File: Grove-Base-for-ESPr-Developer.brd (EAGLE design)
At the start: 26 x 26 mm, 8 parts, among them J1 4P-2.0, J2 4P-2.0, J3 4P-2.0, J4 4P-2.0

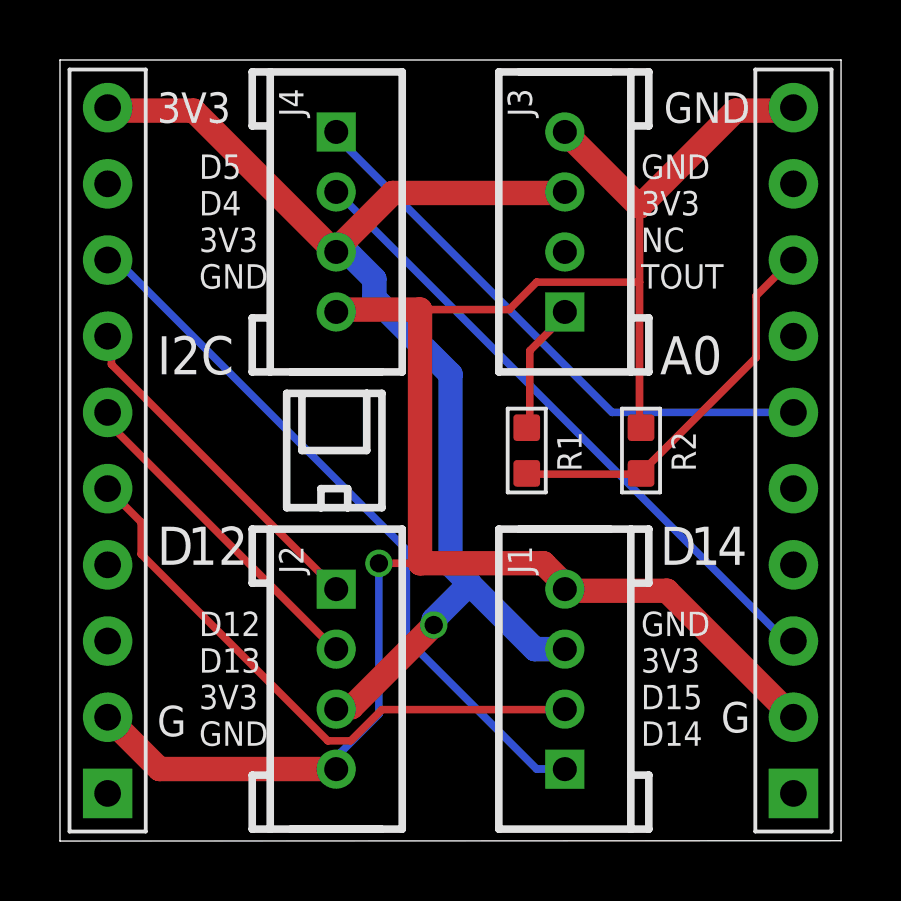
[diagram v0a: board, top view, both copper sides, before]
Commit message: 1st 5V evt
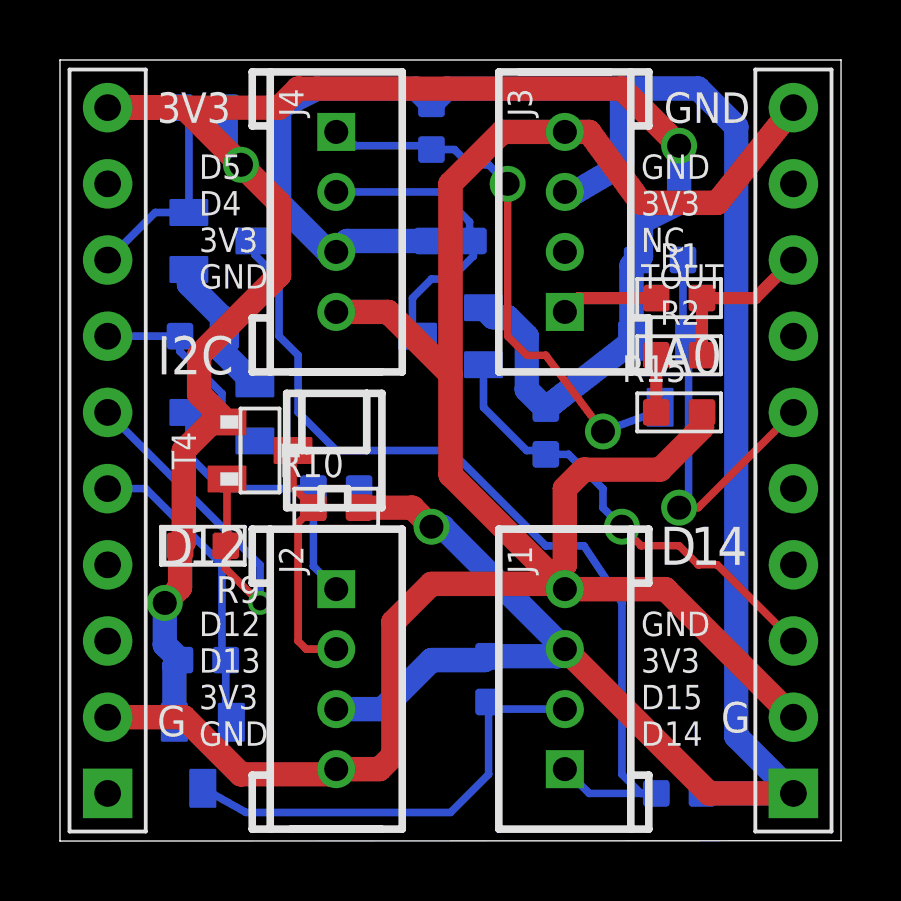
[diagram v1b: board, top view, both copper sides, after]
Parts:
- added R10, R11, R12, R13, R14, R3, R4, R5, R6, R7, R8, R9: 1K, Seeed-OPL-Resistor:R0603
- added R15: 27K, Seeed-OPL-Resistor:R0603
- added T1, T2, T3, T4, T5, T6: (no value), we-transistor:SOT23
- R1: value 220K -> 200K
- R2: value 100K -> 24K
- moved R1 7.18 mm to (20.3, 17.8), turned to 270 degrees
- moved R2 3.42 mm to (20.3, 15.9), turned to 90 degrees
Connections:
- new net IO12_5V: J2.1, R8.1, T3.3
- new net IO13_5V: J2.2, R10.2, T4.3
- new net IO14_5V: J1.1, R4.2, T1.3
- new net IO15_5V: J1.2, R6.2, T2.3
- new net IO4_5V: J4.2, R14.2, T6.3
- new net IO5_5V: J4.1, R12.1, T5.3
- new net N$6: R15.2, R2.1
- net 3V3: now also R11.2, R13.1, R3.1, R5.1, R7.2, R9.1, T1.1, T2.1, T3.1, T4.1, T5.1, T6.1; no longer J1.3, J2.3, J3.3, J4.3
- net 5V: now also J1.3, J2.3, J3.3, J4.3, R10.1, R12.2, R14.1, R4.1, R6.1, R8.2
- net GND: now also R15.1; no longer R2.1
- net IO12: now also R7.1, T3.2; no longer J2.1
- net IO13: now also R9.2, T4.2; no longer J2.2
- net IO14: now also R3.2, T1.2; no longer J1.1
- net IO15: now also R5.2, T2.2; no longer J1.2
- net IO4: now also R13.2, T6.2; no longer J4.2
- net IO5: now also R11.1, T5.2; no longer J4.1
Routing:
- net 5V: track 0.00 -> 82.9 mm, vias 0 -> 1
- net IO14_5V: track 0.00 -> 30.0 mm
- net 3V3: track 41.6 -> 70.8 mm, vias 1 -> 3
- net IO5_5V: track 0.00 -> 18.3 mm, vias 0 -> 2
- net IO14: track 24.2 -> 6.97 mm
- net IO15_5V: track 0.00 -> 15.3 mm
- net IO4_5V: track 0.00 -> 10.0 mm
- net IO12_5V: track 0.00 -> 9.71 mm
- net IO15: track 19.8 -> 10.2 mm
- net IO13_5V: track 0.00 -> 8.22 mm
- net A0: track 13.0 -> 5.48 mm
- net IO4: track 21.6 -> 15.3 mm, vias 0 -> 1
- net GND: track 68.2 -> 74.3 mm, vias 1 -> 0
- net IO5: track 19.2 -> 13.6 mm, vias 0 -> 1
- net IO12: track 11.7 -> 7.03 mm
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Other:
- board text added: "CC: BY-SA K. Hino Sep 29 2016"
- board text removed: "CC: BY-SA S. Kobayashi June 20 2016"
